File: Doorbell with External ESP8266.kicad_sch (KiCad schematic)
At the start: 26 parts, among them J101 Transformer, J102 From Rectifier, J103 To Rectifier, J104 Chime, J105 Button, K101 Relay, Q101 Q_NMOS_GSD, U101 WeMos_D1_mini, U103 EL817

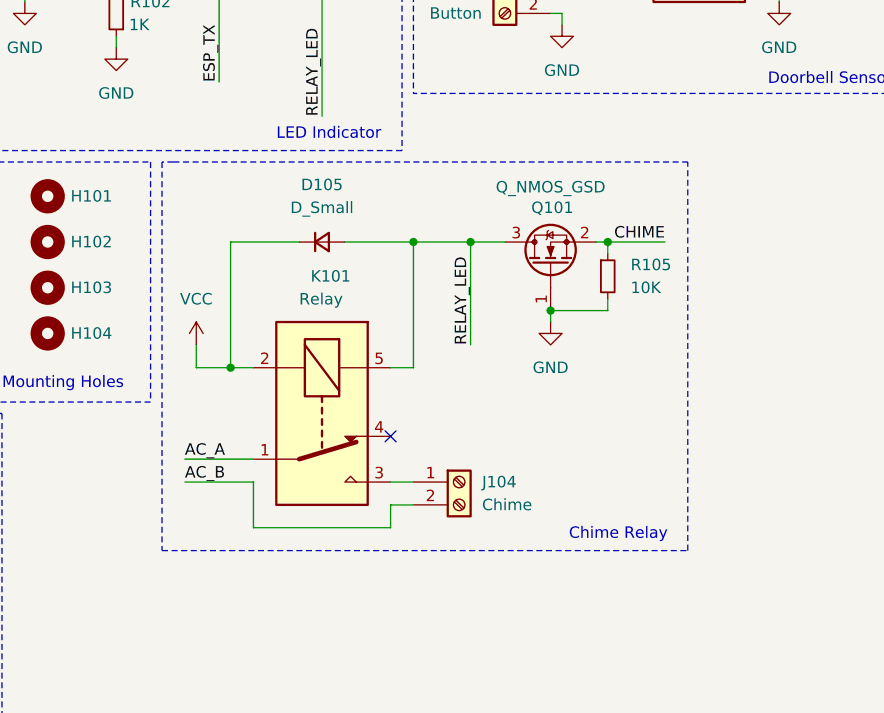
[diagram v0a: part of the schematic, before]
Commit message: schematic fix
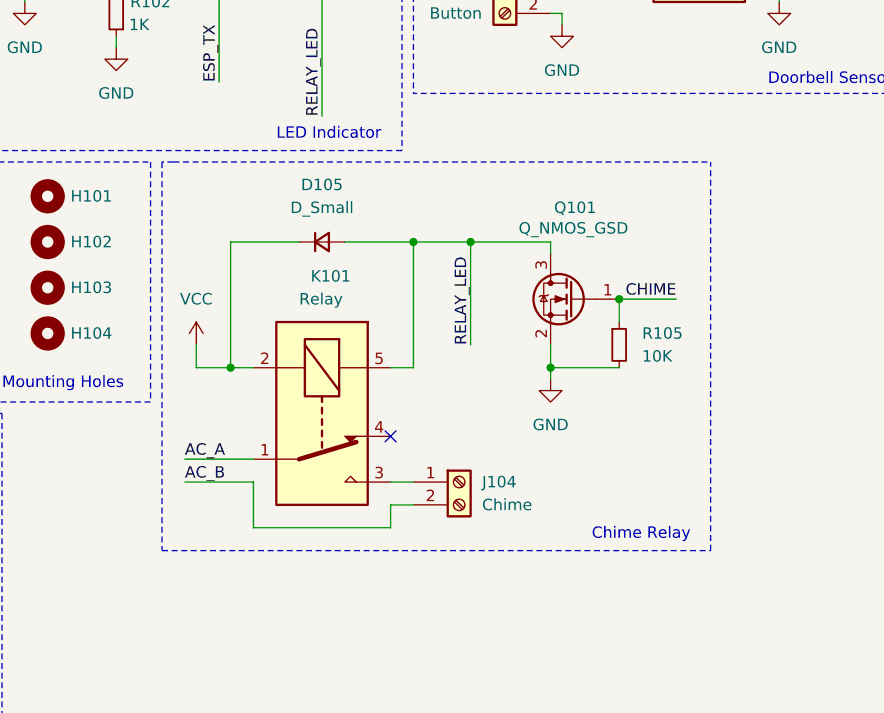
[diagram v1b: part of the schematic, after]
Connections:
- net CHIME: now also Q101.1 (G); no longer Q101.2 (S)
- net GND: now also Q101.2 (S); no longer Q101.1 (G)
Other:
- moved on the sheet: Q101, R105
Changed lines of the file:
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@@
 	)
 	(junction
+		(at 130.81 71.12)
+		(diameter 0)
+		(color 0 0 0 0)
+	)
+	(junction
 		(at 87.63 78.74)
 		(diameter 0)
@@
 	)
 	(junction
-		(at 114.3 64.77)
-		(diameter 0)
-		(color 0 0 0 0)
-	)
-	(junction
 		(at 38.1 111.76)
 		(diameter 0)
@@
 	)
 	(junction
-		(at 129.54 64.77)
+		(at 123.19 78.74)
 		(diameter 0)
 		(color 0 0 0 0)
 	)
 	(junction
-		(at 123.19 72.39)
+		(at 35.56 93.98)
 		(diameter 0)
 		(color 0 0 0 0)
 	)
 	(junction
-		(at 35.56 93.98)
+		(at 114.3 64.77)
 		(diameter 0)
 		(color 0 0 0 0)
@@
 	(wire
 		(pts
-			(xy 129.54 64.77) (xy 135.89 64.77)
+			(xy 130.81 71.12) (xy 137.16 71.12)
 		)
 		(stroke
@@
 	(wire
 		(pts
-			(xy 114.3 64.77) (xy 118.11 64.77)
+			(xy 114.3 64.77) (xy 123.19 64.77)
 		)
 		(stroke
@@
 	(polyline
 		(pts
-			(xy 81.28 55.88) (xy 138.43 55.88)
+			(xy 81.28 55.88) (xy 140.97 55.88)
 		)
 		(stroke
@@
 	(wire
 		(pts
-			(xy 129.54 64.77) (xy 129.54 66.04)
-		)
-		(stroke
-			(width 0)
-			(type default)
-		)
-	)
-	(wire
-		(pts
-			(xy 114.3 76.2) (xy 114.3 64.77)
+			(xy 114.3 64.77) (xy 114.3 76.2)
 		)
 		(stroke
@@
 	(wire
 		(pts
-			(xy 129.54 72.39) (xy 123.19 72.39)
-		)
-		(stroke
-			(width 0)
-			(type default)
-		)
-	)
-	(wire
-		(pts
 			(xy 38.1 106.68) (xy 45.72 106.68)
 		)
@@
 		)
 	)
+	(wire
+		(pts
+			(xy 123.19 78.74) (xy 123.19 80.01)
+		)
+		(stroke
+			(width 0)
+			(type default)
+		)
+	)
 	(polyline
 		(pts
-			(xy 80.01 99.06) (xy 138.43 99.06)
+			(xy 80.01 99.06) (xy 140.97 99.06)
 		)
 		(stroke
@@
 	(wire
 		(pts
-			(xy 123.19 72.39) (xy 123.19 73.66)
+			(xy 123.19 76.2) (xy 123.19 78.74)
 		)
 		(stroke
@@
 	(wire
 		(pts
-			(xy 44.45 45.72) (xy 57.15 45.72)
+			(xy 123.19 64.77) (xy 123.19 66.04)
 		)
 		(stroke
@@
 		)
 	)
-	(polyline
+	(wire
 		(pts
-			(xy 81.28 55.88) (xy 81.28 55.88)
+			(xy 44.45 45.72) (xy 57.15 45.72)
 		)
 		(stroke
 			(width 0)
-			(type dash)
+			(type default)
 		)
 	)
-	(wire
+	(polyline
 		(pts
-			(xy 82.55 91.44) (xy 90.17 91.44)
+			(xy 81.28 55.88) (xy 81.28 55.88)
 		)
 		(stroke
 			(width 0)
-			(type default)
+			(type dash)
 		)
 	)
 	(wire
 		(pts
-			(xy 58.42 106.68) (xy 58.42 105.41)
+			(xy 82.55 91.44) (xy 90.17 91.44)
 		)
 		(stroke
@@
 	(wire
 		(pts
-			(xy 129.54 71.12) (xy 129.54 72.39)
+			(xy 58.42 106.68) (xy 58.42 105.41)
 		)
 		(stroke
@@
 	(wire
 		(pts
+			(xy 130.81 71.12) (xy 130.81 73.66)
+		)
+		(stroke
+			(width 0)
+			(type default)
+		)
+	)
+	(wire
+		(pts
 			(xy 34.29 96.52) (xy 38.1 96.52)
 		)
@@
 	(wire
 		(pts
-			(xy 86.36 36.83) (xy 86.36 46.99)
+			(xy 123.19 78.74) (xy 130.81 78.74)
 		)
 		(stroke
@@
 		)
 	)
-	(polyline
+	(wire
 		(pts
-			(xy 59.69 55.88) (xy 59.69 82.55)
+			(xy 86.36 36.83) (xy 86.36 46.99)
 		)
 		(stroke
 			(width 0)
-			(type dash)
+			(type default)
 		)
 	)
 	(polyline
 		(pts
-			(xy 62.23 83.82) (xy 62.23 120.65)
+			(xy 59.69 55.88) (xy 59.69 82.55)
 		)
 		(stroke
@@
 		)
 	)
-	(wire
+	(polyline
 		(pts
-			(xy 107.95 64.77) (xy 107.95 78.74)
+			(xy 62.23 83.82) (xy 62.23 120.65)
 		)
 		(stroke
 			(width 0)
-			(type default)
+			(type dash)
 		)
 	)
 	(wire
 		(pts
-			(xy 128.27 64.77) (xy 129.54 64.77)
+			(xy 107.95 64.77) (xy 107.95 78.74)
 		)
 		(stroke
@@
 	(polyline
 		(pts
-			(xy 138.43 99.06) (xy 138.43 55.88)
+			(xy 140.97 99.06) (xy 140.97 55.88)
 		)
 		(stroke
@@
 	(text "Chime Relay"
 		(exclude_from_sim no)
-		(at 125.222 98.044 0)
+		(at 127.762 98.044 0)
 		(effects
 			(font
@@
 	)
 	(label "CHIME"
-		(at 135.89 64.77 180)
+		(at 137.16 71.12 180)
 		(fields_autoplaced yes)
 		(effects
@@
 	(symbol
 		(lib_id "Device:Q_NMOS_GSD")
-		(at 123.19 67.31 90)
+		(at 125.73 71.12 0)
+		(mirror y)
 		(unit 1)
 		(exclude_from_sim no)
@@
 		(dnp no)
 		(property "Reference" "Q101"
-			(at 125.73 60.96 90)
+			(at 128.27 60.96 0)
 			(effects
 				(font
@@
 		)
 		(property "Value" "Q_NMOS_GSD"
-			(at 129.286 58.674 90)
+			(at 131.826 63.246 0)
 			(effects
 				(font
@@
 		)
 		(property "Footprint" "Package_TO_SOT_SMD:SOT-23"
-			(at 120.65 62.23 0)
+			(at 120.65 68.58 0)
 			(effects
 				(font
@@
 			)
 		)
-		(property "Datasheet" "~"
-			(at 123.19 67.31 0)
+		(property "Datasheet" "https://wmsc.lcsc.com/wmsc/upload/file/pdf/v2/lcsc/2304140030_Jiangsu-Changjing-Electronics-Technology-Co---Ltd--2N7002_C8545.pdf"
+			(at 125.73 71.12 0)
 			(effects
 				(font
@@
 		)
 		(property "Description" ""
-			(at 123.19 67.31 0)
+			(at 125.73 71.12 0)
 			(effects
 				(font
@@
 		)
 		(property "LCSC" "C8545"
-			(at 123.19 67.31 0)
+			(at 125.73 71.12 0)
+			(effects
+				(font
+					(size 1.27 1.27)
+				)
+				(hide yes)
+			)
+		)
+		(property "Mouser" ""
+			(at 125.73 71.12 0)
 			(effects
 				(font
@@
 	(symbol
 		(lib_id "power:GND")
-		(at 123.19 73.66 0)
+		(at 123.19 80.01 0)
 		(unit 1)
 		(exclude_from_sim no)
@@
 		(fields_autoplaced yes)
 		(property "Reference" "#PWR0112"
-			(at 123.19 80.01 0)
+			(at 123.19 86.36 0)
 			(effects
 				(font
@@
 		)
 		(property "Value" "GND"
-			(at 123.19 78.74 0)
+			(at 123.19 85.09 0)
 			(effects
 				(font
@@
 		)
 		(property "Footprint" ""
-			(at 123.19 73.66 0)
+			(at 123.19 80.01 0)
 			(effects
 				(font
@@
 		)
 		(property "Datasheet" ""
-			(at 123.19 73.66 0)
+			(at 123.19 80.01 0)
 			(effects
 				(font
@@
 		)
 		(property "Description" "Power symbol creates a global label with name \"GND\" , ground"
-			(at 123.19 73.66 0)
+			(at 123.19 80.01 0)
 			(effects
 				(font
@@
 	(symbol
 		(lib_id "Device:R_Small")
-		(at 129.54 68.58 0)
+		(at 130.81 76.2 0)
 		(unit 1)
 		(exclude_from_sim no)
@@
 		(dnp no)
 		(property "Reference" "R105"
-			(at 132.08 67.31 0)
+			(at 133.35 74.93 0)
 			(effects
 				(font
@@
 		)
 		(property "Value" "10K"
-			(at 132.08 69.85 0)
+			(at 133.35 77.47 0)
 			(effects
 				(font
@@
 		)
 		(property "Footprint" "Resistor_SMD:R_0603_1608Metric"
-			(at 129.54 68.58 0)
+			(at 130.81 76.2 0)
 			(effects
 				(font
@@
 		)
 		(property "Datasheet" "~"
-			(at 129.54 68.58 0)
+			(at 130.81 76.2 0)
 			(effects
 				(font
@@
 		)
 		(property "Description" ""
-			(at 129.54 68.58 0)
+			(at 130.81 76.2 0)
 			(effects
 				(font
@@
 		)
 		(property "LCSC" "C25804"
-			(at 129.54 68.58 0)
+			(at 130.81 76.2 0)
 			(effects
 				(font
